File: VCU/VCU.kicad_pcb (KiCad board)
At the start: 2 copper layers, 108 x 38 mm, 28 parts, among them J1 LEMO6, J2 LEMO4, J3 Conn_01x10_Male, J4 Conn_01x04_Male, J5 Conn_Coaxial, U1 EL2140, U2 LM7808_TO220

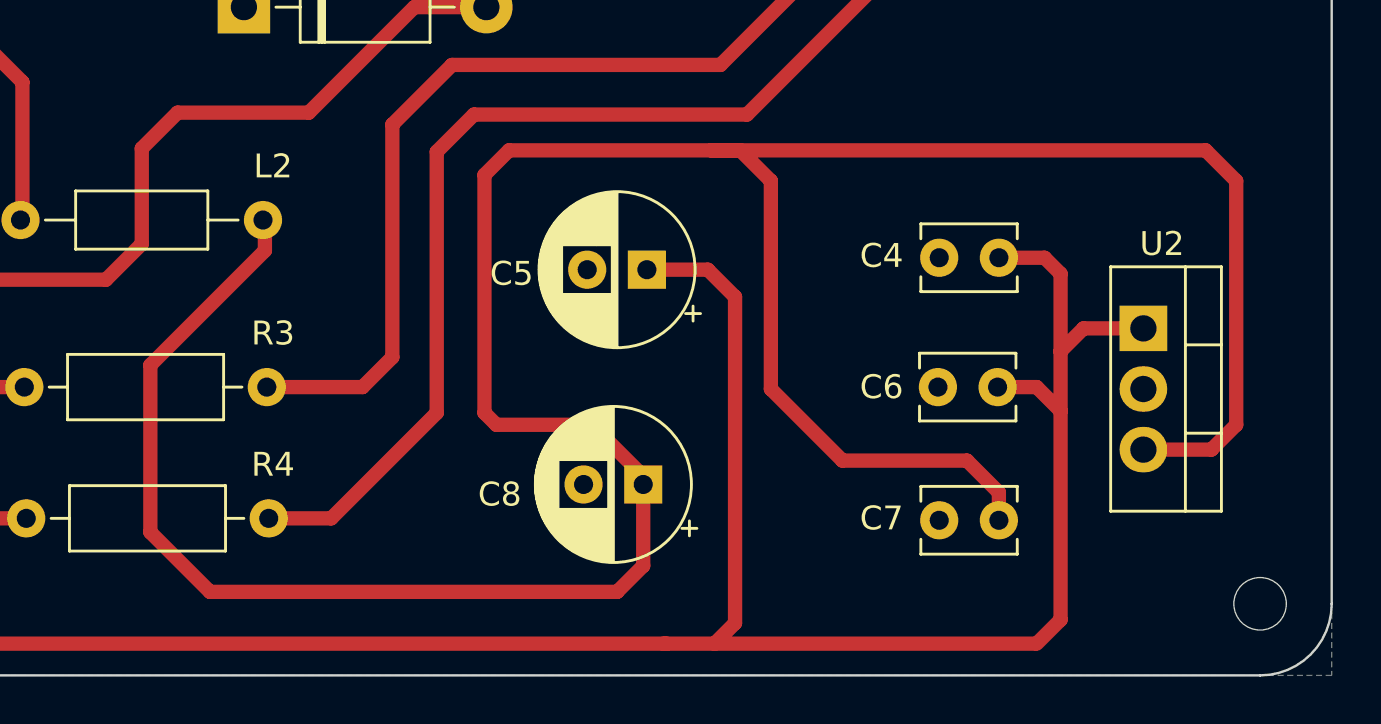
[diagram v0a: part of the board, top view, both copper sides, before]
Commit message: Modifying VCU PCB
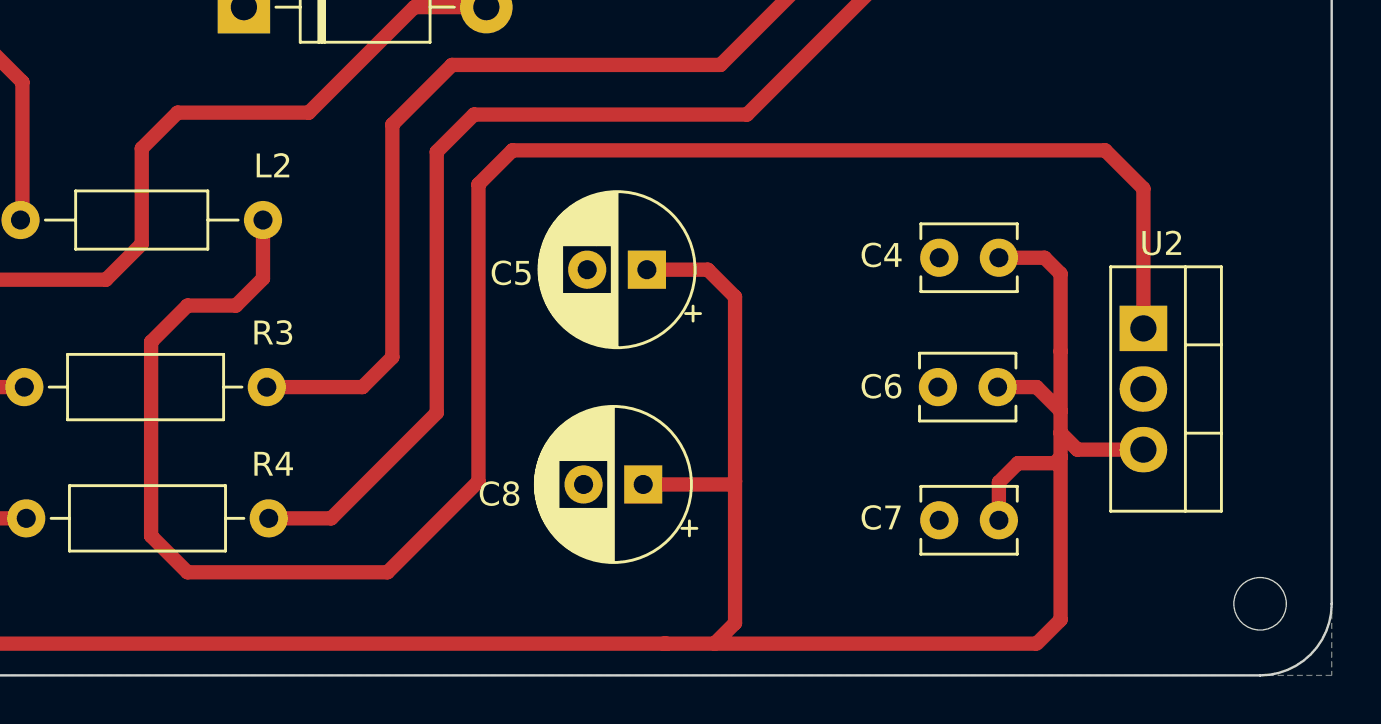
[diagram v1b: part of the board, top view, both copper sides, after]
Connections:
- C7 pad 1: +12V -> +8V
- C8 pad 1: +12V -> +8V
- U2 pad 1: +8V -> +12V
- U2 pad 3: +12V -> +8V
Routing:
- net +12V: track 129.9 -> 79.7 mm
- net +8V: track 154.6 -> 163.3 mm

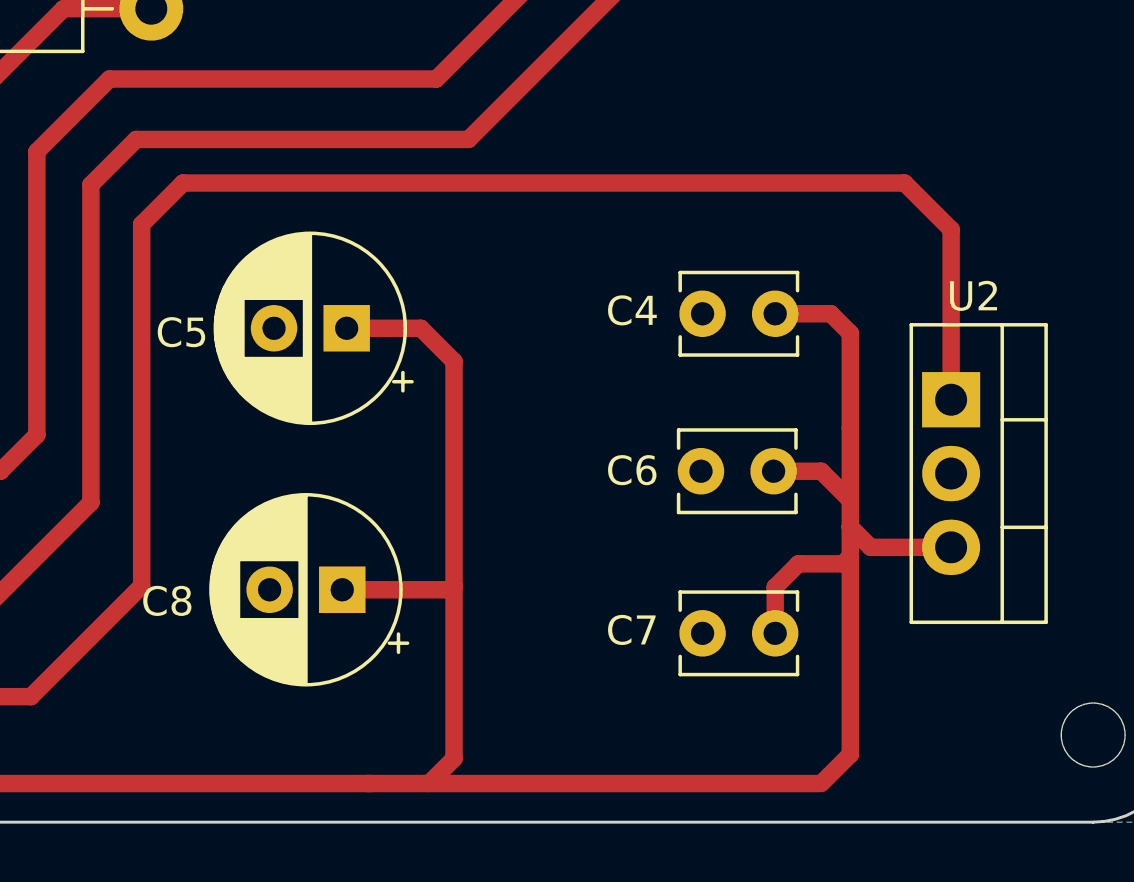
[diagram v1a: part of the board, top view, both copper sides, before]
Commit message: 12V Modifying
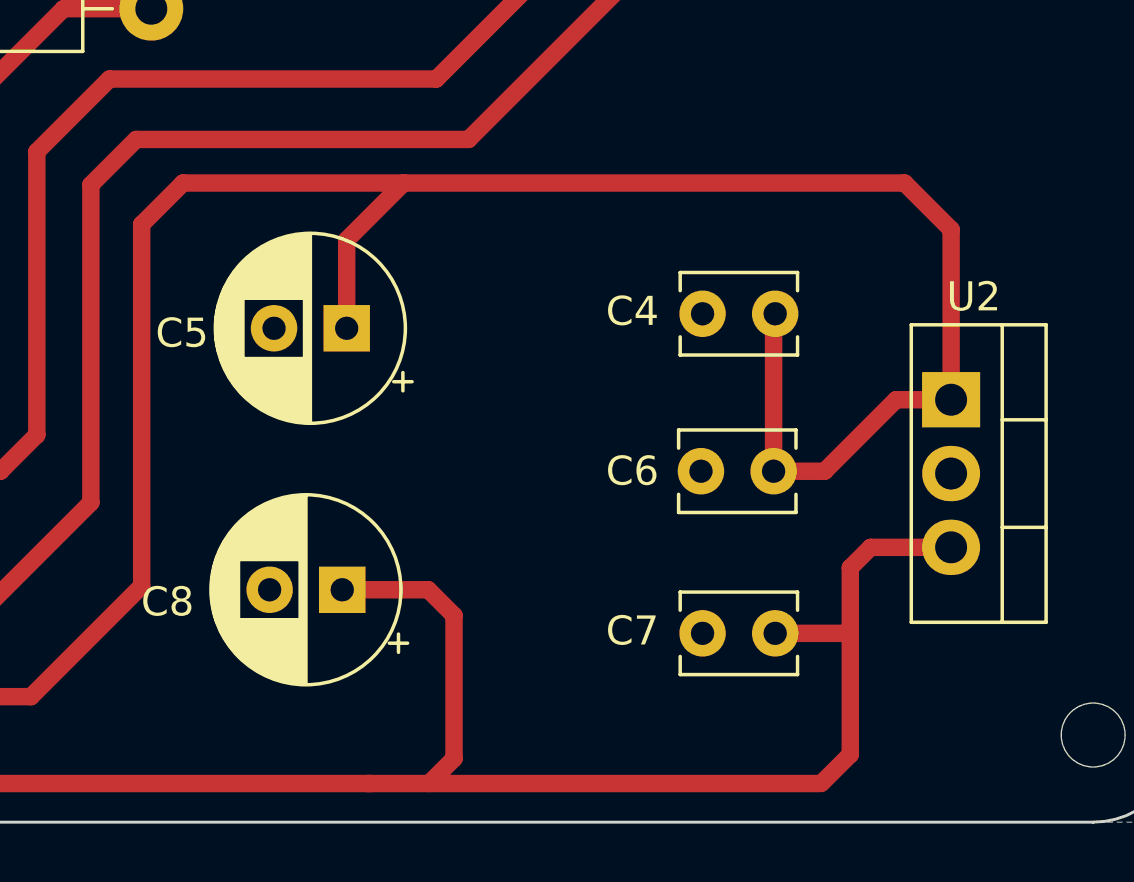
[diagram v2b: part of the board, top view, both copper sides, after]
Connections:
- C4 pad 1: +8V -> 12V
- C5 pad 1: +8V -> 12V
- C6 pad 1: +8V -> 12V
- L2 pad 1: +12V -> 12V
- U2 pad 1: +12V -> 12V
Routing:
- net 12V: track 0.00 -> 98.1 mm
- net +12V: track 79.7 -> 0.00 mm
- net +8V: track 163.3 -> 134.7 mm
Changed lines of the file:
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@@
   (net 4 "Net-(U1-Vinb)")
   (net 5 "+8V")
-  (net 6 "+12V")
+  (net 6 "12V")
   (net 7 "Net-(U1-Vout)")
   (net 8 "Net-(U1-Voutb)")
@@
       (stroke (width 0.1) (type solid)) (layer "F.Fab"))
     (pad "1" thru_hole circle (at 0 0 180) (size 1.6 1.6) (drill 0.8) (layers "*.Cu" "*.Mask")
-      (net 5 "+8V") (pintype "passive"))
+      (net 6 "12V") (pintype "passive"))
     (pad "2" thru_hole circle (at 2.5 0 180) (size 1.6 1.6) (drill 0.8) (layers "*.Cu" "*.Mask")
       (net 3 "GND") (pintype "passive"))
@@
       (stroke (width 0.1) (type solid)) (layer "F.Fab"))
     (pad "1" thru_hole rect (at 0 0 270) (size 1.905 2) (drill 1.1) (layers "*.Cu" "*.Mask")
-      (net 6 "+12V") (pinfunction "VI") (pintype "power_in"))
+      (net 6 "12V") (pinfunction "VI") (pintype "power_in"))
     (pad "2" thru_hole oval (at 2.54 0 270) (size 1.905 2) (drill 1.1) (layers "*.Cu" "*.Mask")
       (net 3 "GND") (pinfunction "GND") (pintype "power_in"))
@@
       (stroke (width 0.1) (type solid)) (layer "F.Fab"))
     (pad "1" thru_hole circle (at 0 0 180) (size 1.6 1.6) (drill 0.8) (layers "*.Cu" "*.Mask")
-      (net 5 "+8V") (pintype "passive"))
+      (net 6 "12V") (pintype "passive"))
     (pad "2" thru_hole circle (at 2.5 0 180) (size 1.6 1.6) (drill 0.8) (layers "*.Cu" "*.Mask")
       (net 3 "GND") (pintype "passive"))
@@
       (stroke (width 0.1) (type solid)) (layer "F.Fab"))
     (pad "1" thru_hole circle (at 0 0 180) (size 1.6 1.6) (drill 0.8) (layers "*.Cu" "*.Mask")
-      (net 6 "+12V") (pinfunction "1") (pintype "passive"))
+      (net 6 "12V") (pinfunction "1") (pintype "passive"))
     (pad "2" thru_hole oval (at 10.16 0 180) (size 1.6 1.6) (drill 0.8) (layers "*.Cu" "*.Mask")
       (net 15 "Net-(J3-Pin_7)") (pinfunction "2") (pintype "passive"))
@@
       (stroke (width 0.1) (type solid)) (fill none) (layer "F.Fab"))
     (pad "1" thru_hole rect (at 0 0 180) (size 1.6 1.6) (drill 0.8) (layers "*.Cu" "*.Mask")
-      (net 5 "+8V") (pintype "passive"))
+      (net 6 "12V") (pintype "passive"))
     (pad "2" thru_hole circle (at 2.5 0 180) (size 1.6 1.6) (drill 0.8) (layers "*.Cu" "*.Mask")
       (net 3 "GND") (pintype "passive"))
@@
   (segment (start 124.66 113) (end 126.36 113) (width 0.6) (layer "F.Cu") (net 4))
   (segment (start 141.24 97) (end 141.24 98.7) (width 0.6) (layer "F.Cu") (net 5))
-  (segment (start 190 106.934) (end 190 113.75) (width 0.6) (layer "F.Cu") (net 5))
-  (segment (start 175.22 99.08) (end 172.665302 99.08) (width 0.6) (layer "F.Cu") (net 5))
-  (segment (start 187.415 107.987) (end 188.214 107.188) (width 0.6) (layer "F.Cu") (net 5))
-  (segment (start 189.746 107.188) (end 190 106.934) (width 0.6) (layer "F.Cu") (net 5))
-  (segment (start 190 102.5) (end 190 99.25) (width 0.6) (layer "F.Cu") (net 5))
-  (segment (start 176.36 107.95) (end 176.36 100.22) (width 0.6) (layer "F.Cu") (net 5))
-  (segment (start 176.23 108.08) (end 176.36 107.95) (width 0.6) (layer "F.Cu") (net 5))
+  (segment (start 189.979 109.58) (end 190 109.601) (width 0.25) (layer "F.Cu") (net 5))
+  (segment (start 176.36 113.89) (end 176.36 108.966) (width 0.6) (layer "F.Cu") (net 5))
   (segment (start 136.86 114.75) (end 115.36 114.75) (width 0.6) (layer "F.Cu") (net 5))
   (segment (start 138.36 108.08) (end 137.36 109.08) (width 0.6) (layer "F.Cu") (net 5))
@@
   (segment (start 141.24 98.7) (end 137.36 102.58) (width 0.6) (layer "F.Cu") (net 5))
   (segment (start 140.98 108.08) (end 138.36 108.08) (width 0.6) (layer "F.Cu") (net 5))
-  (segment (start 187.415 109.58) (end 187.415 107.987) (width 0.6) (layer "F.Cu") (net 5))
   (segment (start 175.5 114.75) (end 176.36 113.89) (width 0.6) (layer "F.Cu") (net 5))
   (segment (start 188.92 114.75) (end 173.36 114.75) (width 0.6) (layer "F.Cu") (net 5))
-  (segment (start 190 105.918) (end 190 106.934) (width 0.6) (layer "F.Cu") (net 5))
-  (segment (start 189 104) (end 190 105) (width 0.6) (layer "F.Cu") (net 5))
+  (segment (start 190 109.601) (end 190 107.322) (width 0.6) (layer "F.Cu") (net 5))
+  (segment (start 190 113.75) (end 190 109.601) (width 0.6) (layer "F.Cu") (net 5))
   (segment (start 137.36 114) (end 136.61 114.75) (width 0.6) (layer "F.Cu") (net 5))
-  (segment (start 172.512651 108.08) (end 176.23 108.08) (width 0.6) (layer "F.Cu") (net 5))
   (segment (start 137.36 102.58) (end 137.36 109.08) (width 0.6) (layer "F.Cu") (net 5))
-  (segment (start 190 105) (end 190 102.5) (width 0.6) (layer "F.Cu") (net 5))
   (segment (start 137 114.75) (end 173.5 114.75) (width 0.6) (layer "F.Cu") (net 5))
-  (segment (start 187.36 104) (end 189 104) (width 0.6) (layer "F.Cu") (net 5))
   (segment (start 190 113.75) (end 189 114.75) (width 0.6) (layer "F.Cu") (net 5))
-  (segment (start 190 105) (end 190 105.918) (width 0.6) (layer "F.Cu") (net 5))
-  (segment (start 190 99.25) (end 189.33 98.58) (width 0.6) (layer "F.Cu") (net 5))
-  (segment (start 176.36 100.22) (end 175.22 99.08) (width 0.6) (layer "F.Cu") (net 5))
+  (segment (start 190 107.322) (end 190.702 106.62) (width 0.6) (layer "F.Cu") (net 5))
   (segment (start 115.36 114.75) (end 114.36 113.75) (width 0.6) (layer "F.Cu") (net 5))
-  (segment (start 190.702 106.62) (end 190 105.918) (width 0.6) (layer "F.Cu") (net 5))
-  (segment (start 188.214 107.188) (end 189.746 107.188) (width 0.6) (layer "F.Cu") (net 5))
+  (segment (start 172.512651 108.08) (end 175.474 108.08) (width 0.6) (layer "F.Cu") (net 5))
   (segment (start 114.94 105) (end 117.08 105) (width 0.6) (layer "F.Cu") (net 5))
-  (segment (start 176.36 113.89) (end 176.36 107.95) (width 0.6) (layer "F.Cu") (net 5))
   (segment (start 172.512651 107.732651) (end 172.512651 108.08) (width 0.6) (layer "F.Cu") (net 5))
   (segment (start 193.47 106.62) (end 190.702 106.62) (width 0.6) (layer "F.Cu") (net 5))
   (segment (start 137.36 109.08) (end 137.36 114) (width 0.6) (layer "F.Cu") (net 5))
-  (segment (start 189.33 98.58) (end 187.415 98.58) (width 0.6) (layer "F.Cu") (net 5))
+  (segment (start 187.415 109.58) (end 189.979 109.58) (width 0.6) (layer "F.Cu") (net 5))
+  (segment (start 175.474 108.08) (end 176.36 108.966) (width 0.6) (layer "F.Cu") (net 5))
   (segment (start 114.36 113.75) (end 114.36 105.58) (width 0.6) (layer "F.Cu") (net 5))
   (segment (start 151.892 102.108) (end 153.416 100.584) (width 0.6) (layer "F.Cu") (net 6))
+  (segment (start 191.87 94.08) (end 174.625 94.08) (width 0.6) (layer "F.Cu") (net 6))
   (segment (start 153.416 111.76) (end 151.892 110.236) (width 0.6) (layer "F.Cu") (net 6))
   (segment (start 156.58 99.452) (end 156.58 97) (width 0.6) (layer "F.Cu") (net 6))
   (segment (start 193.47 95.68) (end 191.87 94.08) (width 0.6) (layer "F.Cu") (net 6))
+  (segment (start 189.116 104) (end 191.576 101.54) (width 0.6) (layer "F.Cu") (net 6))
   (segment (start 161.798 111.76) (end 153.416 111.76) (width 0.6) (layer "F.Cu") (net 6))
   (segment (start 153.416 100.584) (end 155.448 100.584) (width 0.6) (layer "F.Cu") (net 6))
   (segment (start 165.608 95.504) (end 165.608 107.95) (width 0.6) (layer "F.Cu") (net 6))
   (segment (start 165.608 107.95) (end 161.798 111.76) (width 0.6) (layer "F.Cu") (net 6))
+  (segment (start 174.625 94.08) (end 167.032 94.08) (width 0.6) (layer "F.Cu") (net 6))
   (segment (start 167.032 94.08) (end 165.608 95.504) (width 0.6) (layer "F.Cu") (net 6))
   (segment (start 151.892 110.236) (end 151.892 102.108) (width 0.6) (layer "F.Cu") (net 6))
+  (segment (start 172.665302 96.039698) (end 174.625 94.08) (width 0.6) (layer "F.Cu") (net 6))
+  (segment (start 191.576 101.54) (end 193.47 101.54) (width 0.6) (layer "F.Cu") (net 6))
+  (segment (start 172.665302 99.08) (end 172.665302 96.039698) (width 0.6) (layer "F.Cu") (net 6))
   (segment (start 193.47 101.54) (end 193.47 95.68) (width 0.6) (layer "F.Cu") (net 6))
-  (segment (start 191.87 94.08) (end 167.032 94.08) (width 0.6) (layer "F.Cu") (net 6))
   (segment (start 155.448 100.584) (end 156.58 99.452) (width 0.6) (layer "F.Cu") (net 6))
+  (segment (start 187.36 104) (end 189.116 104) (width 0.6) (layer "F.Cu") (net 6))
+  (segment (start 187.36 104) (end 187.36 98.635) (width 0.6) (layer "F.Cu") (net 6))
+  (segment (start 187.36 98.635) (end 187.415 98.58) (width 0.25) (layer "F.Cu") (net 6))
   (segment (start 144.36 104) (end 146.58 104) (width 0.6) (layer "F.Cu") (net 7))
   (segment (start 143.36 103) (end 144.36 104) (width 0.6) (layer "F.Cu") (net 7))
